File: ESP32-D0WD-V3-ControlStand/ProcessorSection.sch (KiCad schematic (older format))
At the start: 50 parts, among them J13 USB_OTG, Q1 UMH3N, SW24 RESET, U10 ESP32-D0WD-V3, U11 W25Q32JVSSIQ, U9 FT231XS-R, Y1 40 Mhz +/- 10 ppm

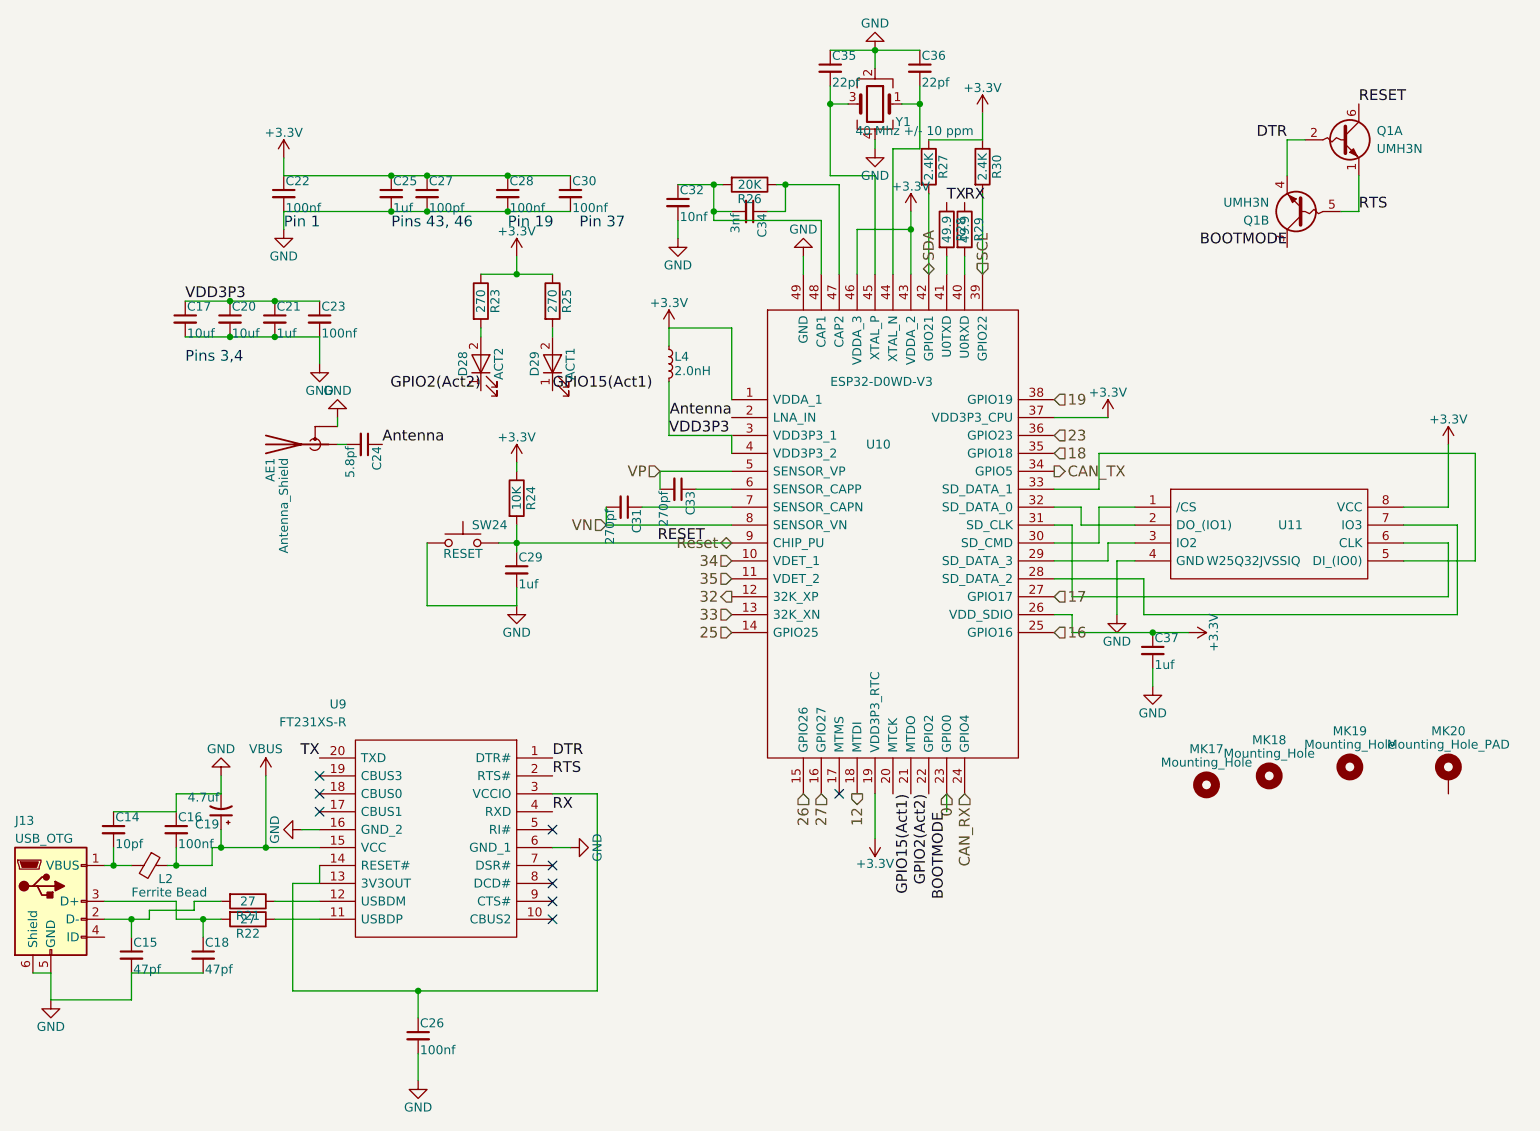
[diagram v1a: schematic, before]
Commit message: Started on V0.1 PCB.
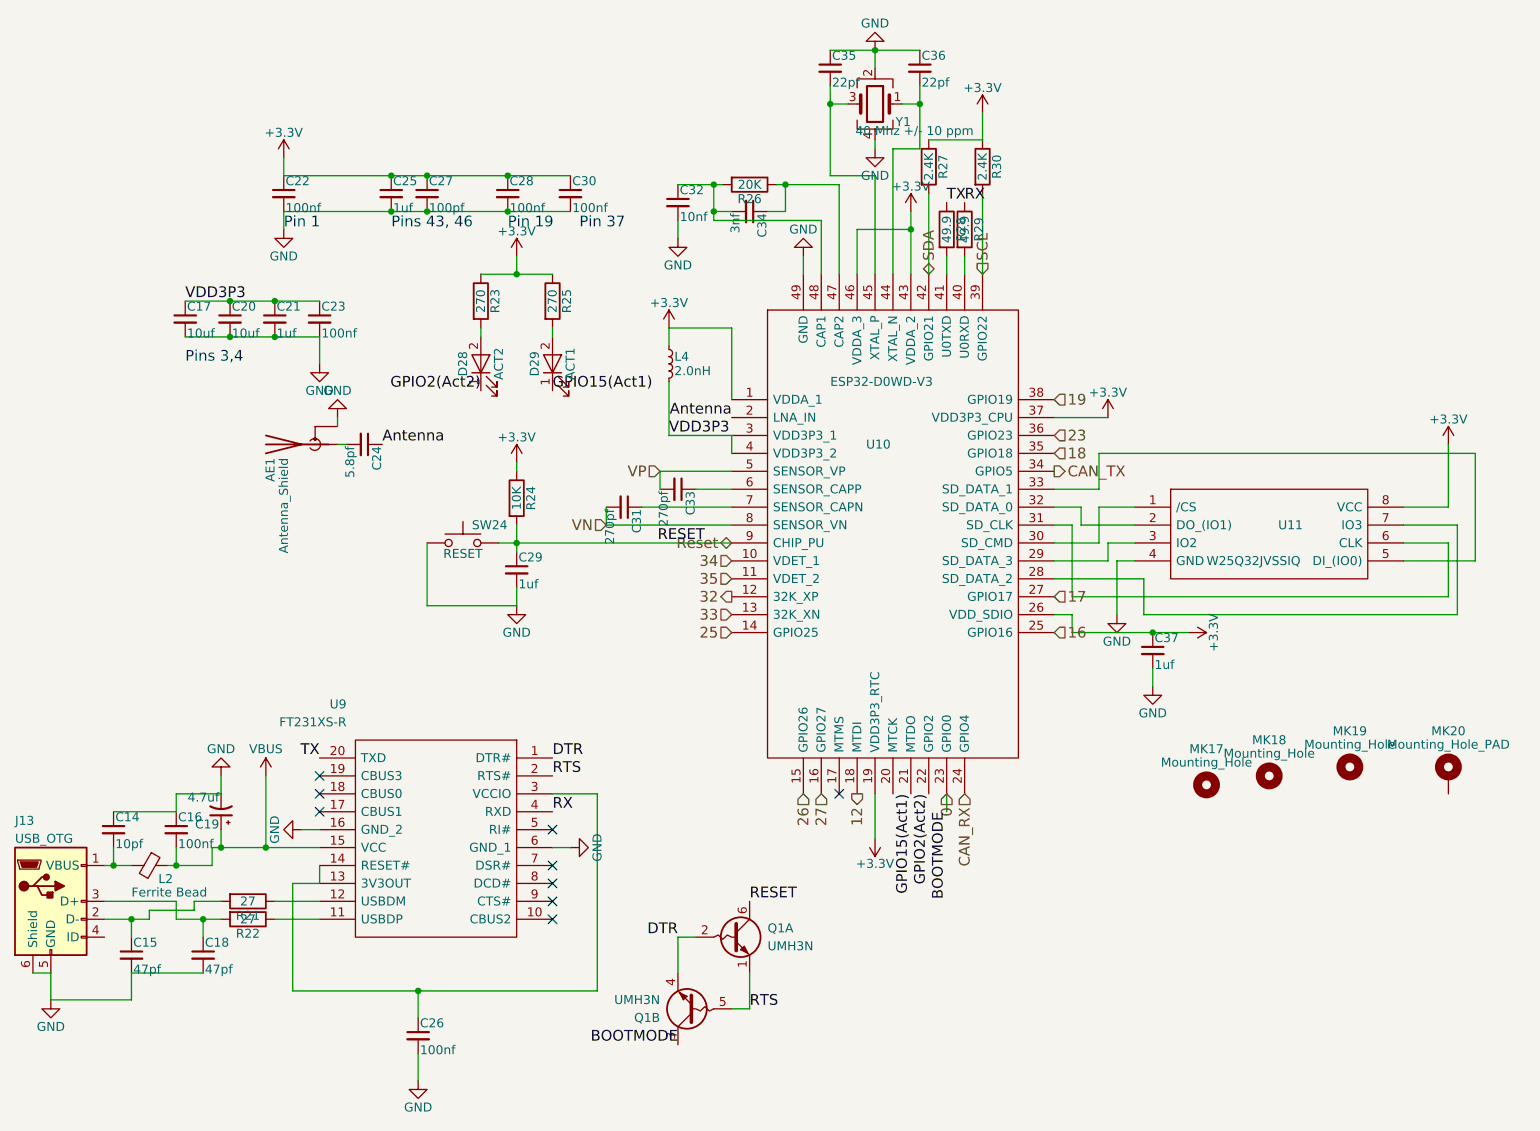
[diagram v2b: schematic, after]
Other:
- moved on the sheet: Q1A, Q1B
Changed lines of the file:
@@
 	1    0    0    -1
 $EndComp
-Text Label 7950 2350 2    60   ~ 0
+Text Label 4550 6800 2    60   ~ 0
 BOOTMODE
 Text Label 6050 5500 3    60   ~ 0
@@
 	6050 5500 6050 5400
 Wire Wire Line
-	3550 4000 4850 4000
+	3550 4000 3650 4000
+Wire Wire Line
+	3650 4000 4850 4000
 Wire Wire Line
 	6150 2400 6150 2500
@@
 	6050 2400 6050 2500
 Wire Wire Line
-	3650 3900 3650 4050
+	3650 3900 3650 4000
+Wire Wire Line
+	3650 4000 3650 4050
 Connection ~ 3650 4000
 Wire Wire Line
@@
 	6750 4400 6750 4500
 Wire Wire Line
-	6750 4500 7400 4500
+	6750 4500 7200 4500
+Wire Wire Line
+	7200 4500 7400 4500
 Wire Wire Line
 	7200 4700 7200 4800
@@
 	4850 2800 4500 2800
 Wire Wire Line
-	5850 2150 5850 2500
+	5850 2150 5850 2250
+Wire Wire Line
+	5850 2250 5850 2500
 Wire Wire Line
 	5850 2250 5550 2250
@@
 	5750 1800 5900 1800
 Wire Wire Line
-	5900 1800 5900 1450
+	5900 1800 5900 1550
+Wire Wire Line
+	5900 1550 5900 1450
 Wire Wire Line
 	5900 1550 5800 1550
@@
 	5650 1950 5400 1950
 Wire Wire Line
-	5400 1950 5400 1450
+	5400 1950 5400 1550
+Wire Wire Line
+	5400 1550 5400 1450
 Wire Wire Line
 	5400 1550 5500 1550
@@
 $EndComp
 Wire Wire Line
-	5400 1250 5900 1250
+	5400 1250 5650 1250
+Wire Wire Line
+	5650 1250 5900 1250
 Connection ~ 5650 1250
 Connection ~ 5900 1550
@@
 	5450 2000 5450 2500
 Wire Wire Line
-	5100 2000 5450 2000
+	5100 2000 5150 2000
+Wire Wire Line
+	5150 2000 5450 2000
 Wire Wire Line
 	5050 2150 5150 2150
@@
 Connection ~ 5150 2000
 Wire Wire Line
-	4550 2000 4800 2000
+	4550 2000 4750 2000
+Wire Wire Line
+	4750 2000 4800 2000
 Wire Wire Line
 	4850 2150 4750 2150
 Wire Wire Line
-	4750 2000 4750 2200
+	4750 2000 4750 2150
+Wire Wire Line
+	4750 2150 4750 2200
 Connection ~ 4750 2000
 Wire Wire Line
@@
 $EndComp
 Wire Wire Line
-	1800 2650 2550 2650
+	1800 2650 2050 2650
+Wire Wire Line
+	2050 2650 2300 2650
+Wire Wire Line
+	2300 2650 2550 2650
 Connection ~ 2300 2650
 Connection ~ 2050 2650
 Wire Wire Line
-	1800 2850 2550 2850
+	1800 2850 2050 2850
+Wire Wire Line
+	2050 2850 2300 2850
+Wire Wire Line
+	2300 2850 2550 2850
 Connection ~ 2300 2850
 Connection ~ 2050 2850
@@
 $EndComp
 Wire Wire Line
-	2350 1950 3950 1950
+	2350 1950 2950 1950
+Wire Wire Line
+	2950 1950 3150 1950
+Wire Wire Line
+	3150 1950 3600 1950
+Wire Wire Line
+	3600 1950 3950 1950
 Connection ~ 3600 1950
 Connection ~ 3150 1950
 Connection ~ 2950 1950
 Wire Wire Line
-	2350 2150 3950 2150
+	2350 2150 2950 2150
+Wire Wire Line
+	2950 2150 3150 2150
+Wire Wire Line
+	3150 2150 3600 2150
+Wire Wire Line
+	3600 2150 3950 2150
 Connection ~ 3600 2150
 Connection ~ 3150 2150
@@
 $EndComp
 Wire Wire Line
-	3850 2500 3450 2500
+	3850 2500 3650 2500
+Wire Wire Line
+	3650 2500 3450 2500
 Wire Wire Line
 	3650 2400 3650 2500
@@
 L UMH3N Q1
 U 1 1 62E11915
-P 8250 1750
-F 0 "Q1" H 8450 1800 50  0000 L CNN
-F 1 "UMH3N" H 8450 1700 50  0000 L CNN
-F 2 "TO_SOT_Packages_SMD:SOT-363_SC-70-6" H 8450 1850 50  0001 C CNN
-F 3 "" H 8250 1750 50  0001 C CNN
-F 4 "755-UMH3NFHATN " H 8250 1750 60  0001 C CNN "Mouser Part Number"
-	1    8250 1750
+P 4850 6200
+F 0 "Q1" H 5050 6250 50  0000 L CNN
+F 1 "UMH3N" H 5050 6150 50  0000 L CNN
+F 2 "TO_SOT_Packages_SMD:SOT-363_SC-70-6" H 5050 6300 50  0001 C CNN
+F 3 "" H 4850 6200 50  0001 C CNN
+F 4 "755-UMH3NFHATN " H 4850 6200 60  0001 C CNN "Mouser Part Number"
+	1    4850 6200
 	1    0    0    -1
 $EndComp
@@
 L UMH3N Q1
 U 2 1 62E14AAD
-P 8050 2150
-F 0 "Q1" H 8250 2200 50  0000 L CNN
-F 1 "UMH3N" H 8250 2100 50  0000 L CNN
-F 2 "TO_SOT_Packages_SMD:SOT-363_SC-70-6" H 8250 2250 50  0001 C CNN
-F 3 "" H 8050 2150 50  0001 C CNN
-F 4 "755-UMH3NFHATN " H 8050 2150 60  0001 C CNN "Mouser Part Number"
-	2    8050 2150
+P 4650 6600
+F 0 "Q1" H 4850 6650 50  0000 L CNN
+F 1 "UMH3N" H 4850 6550 50  0000 L CNN
+F 2 "TO_SOT_Packages_SMD:SOT-363_SC-70-6" H 4850 6700 50  0001 C CNN
+F 3 "" H 4650 6600 50  0001 C CNN
+F 4 "755-UMH3NFHATN " H 4650 6600 60  0001 C CNN "Mouser Part Number"
+	2    4650 6600
 	-1   0    0    1
 $EndComp
 Wire Wire Line
-	8350 1950 8350 2150
-Wire Wire Line
-	8350 2150 8250 2150
-Wire Wire Line
-	8050 1750 7950 1750
-Wire Wire Line
-	7950 1750 7950 1950
-Text Label 8350 1550 0    60   ~ 0
+	4950 6400 4950 6600
+Wire Wire Line
+	4950 6600 4850 6600
+Wire Wire Line
+	4650 6200 4550 6200
+Wire Wire Line
+	4550 6200 4550 6400
+Text Label 4950 6000 0    60   ~ 0
 RESET
-Text Label 7950 1750 2    60   ~ 0
+Text Label 4550 6200 2    60   ~ 0
 DTR
-Text Label 8350 2150 0    60   ~ 0
+Text Label 4950 6600 0    60   ~ 0
 RTS
 Text Label 3850 5200 0    60   ~ 0
@@
 	1750 6000 1750 6100
 Wire Wire Line
-	1750 6100 2000 6100
+	1750 6100 1900 6100
+Wire Wire Line
+	1900 6100 2000 6100
 Wire Wire Line
 	2300 6100 2550 6100
@@
 	2300 6000 2550 6000
 Wire Wire Line
-	1350 6100 1600 6100
+	1350 6100 1500 6100
+Wire Wire Line
+	1500 6100 1600 6100
 Wire Wire Line
 	1600 6100 1600 6050
@@
 $EndComp
 Wire Wire Line
-	1350 5800 1500 5800
-Wire Wire Line
-	2550 5700 1950 5700
+	1350 5800 1400 5800
+Wire Wire Line
+	1400 5800 1500 5800
+Wire Wire Line
+	2550 5700 2250 5700
+Wire Wire Line
+	2250 5700 2000 5700
+Wire Wire Line
+	2000 5700 1950 5700
 Wire Wire Line
 	1950 5700 1950 5800
 Wire Wire Line
-	1950 5800 1700 5800
+	1950 5800 1750 5800
+Wire Wire Line
+	1750 5800 1700 5800
 Wire Wire Line
 	2550 5800 2550 5900
@@
 	2400 5900 2400 6500
 Wire Wire Line
-	2400 6500 4100 6500
+	2400 6500 3100 6500
+Wire Wire Line
+	3100 6500 4100 6500
 Wire Wire Line
 	4100 6500 4100 5400

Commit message: About halfway done.
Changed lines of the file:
@@
 $EndComp
 $Comp
-L +3.3V #PWR062
+L +3.3V #PWR060
 U 1 1 62DF2387
 P 8850 3450
-F 0 "#PWR062" H 8850 3300 50  0001 C CNN
+F 0 "#PWR060" H 8850 3300 50  0001 C CNN
 F 1 "+3.3V" H 8850 3590 50  0000 C CNN
 F 2 "" H 8850 3450 50  0001 C CNN
@@
 $EndComp
 $Comp
-L GND #PWR063
+L GND #PWR061
 U 1 1 62DF2388
 P 7000 4400
-F 0 "#PWR063" H 7000 4150 50  0001 C CNN
+F 0 "#PWR061" H 7000 4150 50  0001 C CNN
 F 1 "GND" H 7000 4250 50  0000 C CNN
 F 2 "" H 7000 4400 50  0001 C CNN
@@
 $EndComp
 $Comp
-L GND #PWR064
+L GND #PWR062
 U 1 1 62DF2391
 P 3650 4350
-F 0 "#PWR064" H 3650 4100 50  0001 C CNN
+F 0 "#PWR062" H 3650 4100 50  0001 C CNN
 F 1 "GND" H 3650 4200 50  0000 C CNN
 F 2 "" H 3650 4350 50  0001 C CNN
@@
 $EndComp
 $Comp
-L +3.3V #PWR065
+L +3.3V #PWR063
 U 1 1 62DF2392
 P 3650 3550
-F 0 "#PWR065" H 3650 3400 50  0001 C CNN
+F 0 "#PWR063" H 3650 3400 50  0001 C CNN
 F 1 "+3.3V" H 3650 3690 50  0000 C CNN
 F 2 "" H 3650 3550 50  0001 C CNN
@@
 $EndComp
 $Comp
-L GND #PWR066
+L GND #PWR064
 U 1 1 62DF2394
 P 7200 4800
-F 0 "#PWR066" H 7200 4550 50  0001 C CNN
+F 0 "#PWR064" H 7200 4550 50  0001 C CNN
 F 1 "GND" H 7200 4650 50  0000 C CNN
 F 2 "" H 7200 4800 50  0001 C CNN
@@
 $EndComp
 $Comp
-L +3.3V #PWR067
+L +3.3V #PWR065
 U 1 1 62DF2395
 P 7400 4500
-F 0 "#PWR067" H 7400 4350 50  0001 C CNN
+F 0 "#PWR065" H 7400 4350 50  0001 C CNN
 F 1 "+3.3V" H 7400 4640 50  0000 C CNN
 F 2 "" H 7400 4500 50  0001 C CNN
@@
 $EndComp
 $Comp
-L +3.3V #PWR068
+L +3.3V #PWR066
 U 1 1 62DF2397
 P 4500 2800
-F 0 "#PWR068" H 4500 2650 50  0001 C CNN
+F 0 "#PWR066" H 4500 2650 50  0001 C CNN
 F 1 "+3.3V" H 4500 2940 50  0000 C CNN
 F 2 "" H 4500 2800 50  0001 C CNN
@@
 $EndComp
 $Comp
-L +3.3V #PWR069
+L +3.3V #PWR067
 U 1 1 62DF2398
 P 6950 3300
-F 0 "#PWR069" H 6950 3150 50  0001 C CNN
+F 0 "#PWR067" H 6950 3150 50  0001 C CNN
 F 1 "+3.3V" H 6950 3440 50  0000 C CNN
 F 2 "" H 6950 3300 50  0001 C CNN
@@
 $EndComp
 $Comp
-L +3.3V #PWR070
+L +3.3V #PWR068
 U 1 1 62DF2399
 P 5850 2150
-F 0 "#PWR070" H 5850 2000 50  0001 C CNN
+F 0 "#PWR068" H 5850 2000 50  0001 C CNN
 F 1 "+3.3V" H 5850 2290 50  0000 C CNN
 F 2 "" H 5850 2150 50  0001 C CNN
@@
 $EndComp
 $Comp
-L +3.3V #PWR071
+L +3.3V #PWR069
 U 1 1 62DF239A
 P 5650 5650
-F 0 "#PWR071" H 5650 5500 50  0001 C CNN
+F 0 "#PWR069" H 5650 5500 50  0001 C CNN
 F 1 "+3.3V" H 5650 5790 50  0000 C CNN
 F 2 "" H 5650 5650 50  0001 C CNN
@@
 VDD3P3
 $Comp
-L GND #PWR072
+L GND #PWR070
 U 1 1 62DF239B
 P 5250 2400
-F 0 "#PWR072" H 5250 2150 50  0001 C CNN
+F 0 "#PWR070" H 5250 2150 50  0001 C CNN
 F 1 "GND" H 5250 2250 50  0000 C CNN
 F 2 "" H 5250 2400 50  0001 C CNN
@@
 	6050 5500 6050 5400
 Wire Wire Line
-	3550 4000 3650 4000
-Wire Wire Line
-	3650 4000 4850 4000
+	3550 4000 4850 4000
 Wire Wire Line
 	6150 2400 6150 2500
@@
 	6050 2400 6050 2500
 Wire Wire Line
-	3650 3900 3650 4000
-Wire Wire Line
-	3650 4000 3650 4050
+	3650 3900 3650 4050
 Connection ~ 3650 4000
 Wire Wire Line
@@
 	6750 4400 6750 4500
 Wire Wire Line
-	6750 4500 7200 4500
-Wire Wire Line
-	7200 4500 7400 4500
+	6750 4500 7400 4500
 Wire Wire Line
 	7200 4700 7200 4800
@@
 	4850 2800 4500 2800
 Wire Wire Line
-	5850 2150 5850 2250
-Wire Wire Line
-	5850 2250 5850 2500
+	5850 2150 5850 2500
 Wire Wire Line
 	5850 2250 5550 2250
@@
 	5750 1800 5900 1800
 Wire Wire Line
-	5900 1800 5900 1550
-Wire Wire Line
-	5900 1550 5900 1450
+	5900 1800 5900 1450
 Wire Wire Line
 	5900 1550 5800 1550
@@
 	5650 1950 5400 1950
 Wire Wire Line
-	5400 1950 5400 1550
-Wire Wire Line
-	5400 1550 5400 1450
+	5400 1950 5400 1450
 Wire Wire Line
 	5400 1550 5500 1550
 $Comp
-L GND #PWR073
+L GND #PWR071
 U 1 1 62DF239D
 P 5650 1800
-F 0 "#PWR073" H 5650 1550 50  0001 C CNN
+F 0 "#PWR071" H 5650 1550 50  0001 C CNN
 F 1 "GND" H 5650 1650 50  0000 C CNN
 F 2 "" H 5650 1800 50  0001 C CNN
@@
 $EndComp
 $Comp
-L GND #PWR074
+L GND #PWR072
 U 1 1 62DF239E
 P 5650 1250
-F 0 "#PWR074" H 5650 1000 50  0001 C CNN
+F 0 "#PWR072" H 5650 1000 50  0001 C CNN
 F 1 "GND" H 5650 1100 50  0000 C CNN
 F 2 "" H 5650 1250 50  0001 C CNN
@@
 $EndComp
 Wire Wire Line
-	5400 1250 5650 1250
-Wire Wire Line
-	5650 1250 5900 1250
+	5400 1250 5900 1250
 Connection ~ 5650 1250
 Connection ~ 5900 1550
@@
 	5450 2000 5450 2500
 Wire Wire Line
-	5100 2000 5150 2000
-Wire Wire Line
-	5150 2000 5450 2000
+	5100 2000 5450 2000
 Wire Wire Line
 	5050 2150 5150 2150
@@
 Connection ~ 5150 2000
 Wire Wire Line
-	4550 2000 4750 2000
-Wire Wire Line
-	4750 2000 4800 2000
+	4550 2000 4800 2000
 Wire Wire Line
 	4850 2150 4750 2150
 Wire Wire Line
-	4750 2000 4750 2150
-Wire Wire Line
-	4750 2150 4750 2200
+	4750 2000 4750 2200
 Connection ~ 4750 2000
 Wire Wire Line
@@
 Connection ~ 4750 2150
 $Comp
-L GND #PWR075
+L GND #PWR073
 U 1 1 62DF23A4
 P 4550 2300
-F 0 "#PWR075" H 4550 2050 50  0001 C CNN
+F 0 "#PWR073" H 4550 2050 50  0001 C CNN
 F 1 "GND" H 4550 2150 50  0000 C CNN
 F 2 "" H 4550 2300 50  0001 C CNN
@@
 $EndComp
 Wire Wire Line
-	1800 2650 2050 2650
-Wire Wire Line
-	2050 2650 2300 2650
-Wire Wire Line
-	2300 2650 2550 2650
+	1800 2650 2550 2650
 Connection ~ 2300 2650
 Connection ~ 2050 2650
 Wire Wire Line
-	1800 2850 2050 2850
-Wire Wire Line
-	2050 2850 2300 2850
-Wire Wire Line
-	2300 2850 2550 2850
+	1800 2850 2550 2850
 Connection ~ 2300 2850
 Connection ~ 2050 2850
 $Comp
-L GND #PWR076
+L GND #PWR074
 U 1 1 62DF23A9
 P 2550 3000
-F 0 "#PWR076" H 2550 2750 50  0001 C CNN
+F 0 "#PWR074" H 2550 2750 50  0001 C CNN
 F 1 "GND" H 2550 2850 50  0000 C CNN
 F 2 "" H 2550 3000 50  0001 C CNN
@@
 $EndComp
 Wire Wire Line
-	2350 1950 2950 1950
-Wire Wire Line
-	2950 1950 3150 1950
-Wire Wire Line
-	3150 1950 3600 1950
-Wire Wire Line
-	3600 1950 3950 1950
+	2350 1950 3950 1950
 Connection ~ 3600 1950
 Connection ~ 3150 1950
 Connection ~ 2950 1950
 Wire Wire Line
-	2350 2150 2950 2150
-Wire Wire Line
-	2950 2150 3150 2150
-Wire Wire Line
-	3150 2150 3600 2150
-Wire Wire Line
-	3600 2150 3950 2150
+	2350 2150 3950 2150
 Connection ~ 3600 2150
 Connection ~ 3150 2150
 Connection ~ 2950 2150
 $Comp
-L +3.3V #PWR077
+L +3.3V #PWR075
 U 1 1 62DF23AF
 P 2350 1850
-F 0 "#PWR077" H 2350 1700 50  0001 C CNN
+F 0 "#PWR075" H 2350 1700 50  0001 C CNN
 F 1 "+3.3V" H 2350 1990 50  0000 C CNN
 F 2 "" H 2350 1850 50  0001 C CNN
@@
 $EndComp
 $Comp
-L GND #PWR078
+L GND #PWR076
 U 1 1 62DF23B0
 P 2350 2250
-F 0 "#PWR078" H 2350 2000 50  0001 C CNN
+F 0 "#PWR076" H 2350 2000 50  0001 C CNN
 F 1 "GND" H 2350 2100 50  0000 C CNN
 F 2 "" H 2350 2250 50  0001 C CNN
@@
 	5950 1750 6250 1750
 $Comp
-L +3.3V #PWR079
+L +3.3V #PWR077
 U 1 1 62DF23B3
 P 6250 1600
-F 0 "#PWR079" H 6250 1450 50  0001 C CNN
+F 0 "#PWR077" H 6250 1450 50  0001 C CNN
 F 1 "+3.3V" H 6250 1740 50  0000 C CNN
 F 2 "" H 6250 1600 50  0001 C CNN
@@
 $EndComp
 $Comp
-L +3.3V #PWR080
+L +3.3V #PWR078
 U 1 1 62DF23B8
 P 3650 2400
-F 0 "#PWR080" H 3650 2250 50  0001 C CNN
+F 0 "#PWR078" H 3650 2250 50  0001 C CNN
 F 1 "+3.3V" H 3650 2540 50  0000 C CNN
 F 2 "" H 3650 2400 50  0001 C CNN
@@
 $EndComp
 Wire Wire Line
-	3850 2500 3650 2500
-Wire Wire Line
-	3650 2500 3450 2500
+	3450 2500 3850 2500
 Wire Wire Line
 	3650 2400 3650 2500
@@
 NoConn ~ 3850 6000
 $Comp
-L GND #PWR081
+L GND #PWR079
 U 1 1 62E17368
 P 3950 5700
-F 0 "#PWR081" H 3950 5450 50  0001 C CNN
+F 0 "#PWR079" H 3950 5450 50  0001 C CNN
 F 1 "GND" H 3950 5550 50  0000 C CNN
 F 2 "" H 3950 5700 50  0001 C CNN
@@
 NoConn ~ 2550 5300
 $Comp
-L GND #PWR082
+L GND #PWR080
 U 1 1 62E179B5
 P 2450 5600
-F 0 "#PWR082" H 2450 5350 50  0001 C CNN
+F 0 "#PWR080" H 2450 5350 50  0001 C CNN
 F 1 "GND" H 2450 5450 50  0000 C CNN
 F 2 "" H 2450 5600 50  0001 C CNN
@@
 	1750 6000 1750 6100
 Wire Wire Line
-	1750 6100 1900 6100
-Wire Wire Line
-	1900 6100 2000 6100
+	1750 6100 2000 6100
 Wire Wire Line
 	2300 6100 2550 6100
@@
 	2300 6000 2550 6000
 Wire Wire Line
-	1350 6100 1500 6100
-Wire Wire Line
-	1500 6100 1600 6100
+	1350 6100 1600 6100
 Wire Wire Line
 	1600 6100 1600 6050
@@
 	950  6400 1050 6400
 $Comp
-L GND #PWR083
+L GND #PWR081
 U 1 1 62E187A2
 P 1050 6550
-F 0 "#PWR083" H 1050 6300 50  0001 C CNN
+F 0 "#PWR081" H 1050 6300 50  0001 C CNN
 F 1 "GND" H 1050 6400 50  0000 C CNN
 F 2 "" H 1050 6550 50  0001 C CNN
@@
 $EndComp
 Wire Wire Line
-	1350 5800 1400 5800
-Wire Wire Line
-	1400 5800 1500 5800
-Wire Wire Line
-	2550 5700 2250 5700
-Wire Wire Line
-	2250 5700 2000 5700
-Wire Wire Line
-	2000 5700 1950 5700
-Wire Wire Line
-	1950 5700 1950 5800
-Wire Wire Line
-	1950 5800 1750 5800
-Wire Wire Line
-	1750 5800 1700 5800
+	1350 5800 1500 5800
+Wire Wire Line
+	1950 5700 2550 5700
+Wire Wire Line
+	1950 5800 1950 5700
+Wire Wire Line
+	1700 5800 1950 5800
 Wire Wire Line
 	2550 5800 2550 5900
@@
 	2400 5900 2400 6500
 Wire Wire Line
-	2400 6500 3100 6500
-Wire Wire Line
-	3100 6500 4100 6500
+	2400 6500 4100 6500
 Wire Wire Line
 	4100 6500 4100 5400
@@
 	1750 5400 2000 5400
 $Comp
-L GND #PWR084
+L GND #PWR082
 U 1 1 62E1A0F6
 P 2000 5300
-F 0 "#PWR084" H 2000 5050 50  0001 C CNN
+F 0 "#PWR082" H 2000 5050 50  0001 C CNN
 F 1 "GND" H 2000 5150 50  0000 C CNN
 F 2 "" H 2000 5300 50  0001 C CNN
@@
 Connection ~ 3100 6500
 $Comp
-L GND #PWR085
+L GND #PWR083
 U 1 1 62E1A448
 P 3100 7000
-F 0 "#PWR085" H 3100 6750 50  0001 C CNN
+F 0 "#PWR083" H 3100 6750 50  0001 C CNN
 F 1 "GND" H 3100 6850 50  0000 C CNN
 F 2 "" H 3100 7000 50  0001 C CNN
@@
 	2700 3450 2650 3450
 $Comp
-L GND #PWR086
+L GND #PWR084
 U 1 1 62E1EC1A
 P 2650 3300
-F 0 "#PWR086" H 2650 3050 50  0001 C CNN
+F 0 "#PWR084" H 2650 3050 50  0001 C CNN
 F 1 "GND" H 2650 3150 50  0000 C CNN
 F 2 "" H 2650 3300 50  0001 C CNN
@@
 	2650 3300 2650 3350
 $Comp
-L VBUS #PWR087
+L VBUS #PWR085
 U 1 1 62E2A6A1
 P 2250 5300
-F 0 "#PWR087" H 2250 5150 50  0001 C CNN
+F 0 "#PWR085" H 2250 5150 50  0001 C CNN
 F 1 "VBUS" H 2250 5450 50  0000 C CNN
 F 2 "" H 2250 5300 50  0001 C CNN
